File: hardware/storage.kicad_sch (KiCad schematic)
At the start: 2 parts, among them J3 Micro_SD_Card

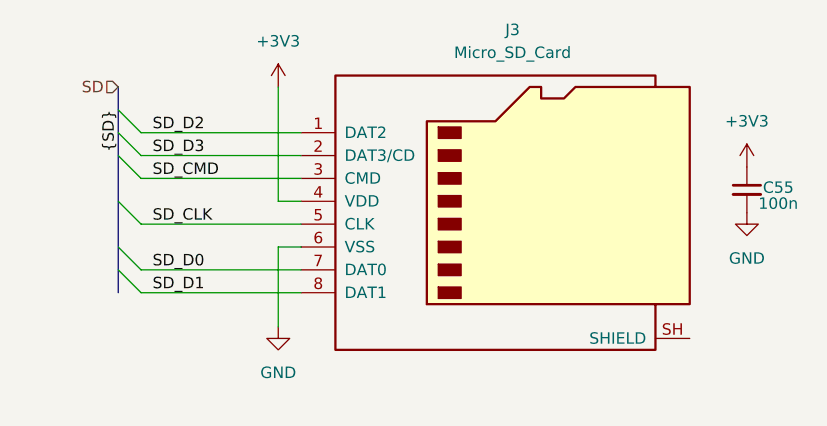
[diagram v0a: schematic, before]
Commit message: final touches
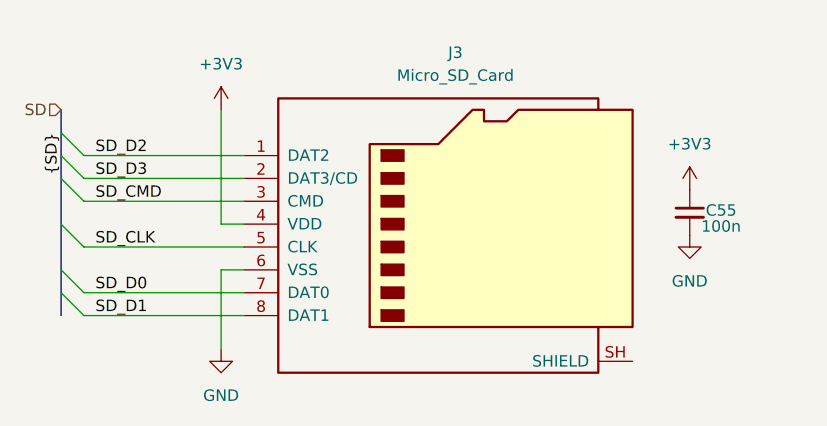
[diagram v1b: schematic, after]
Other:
- moved on the sheet: C55, J3
